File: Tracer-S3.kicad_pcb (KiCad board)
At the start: 2 copper layers, 92.7 x 86.8 mm, 41 parts, among them J1 Conn_01x06_Socket, J2 Conn_02x02_Odd_Even, J3 Conn_02x02_Odd_Even, J4 Conn_02x02_Odd_Even, J5 Conn_02x02_Odd_Even, J6 Conn_02x04_Odd_Even, J7 Conn_01x02_Pin, Q1 BSP89, SW1 SW_Push, SW2 SW_Push, SW3 SW_SPDT, U1 ESP32-S3-WROOM-1, U2 AMS1117-3.3

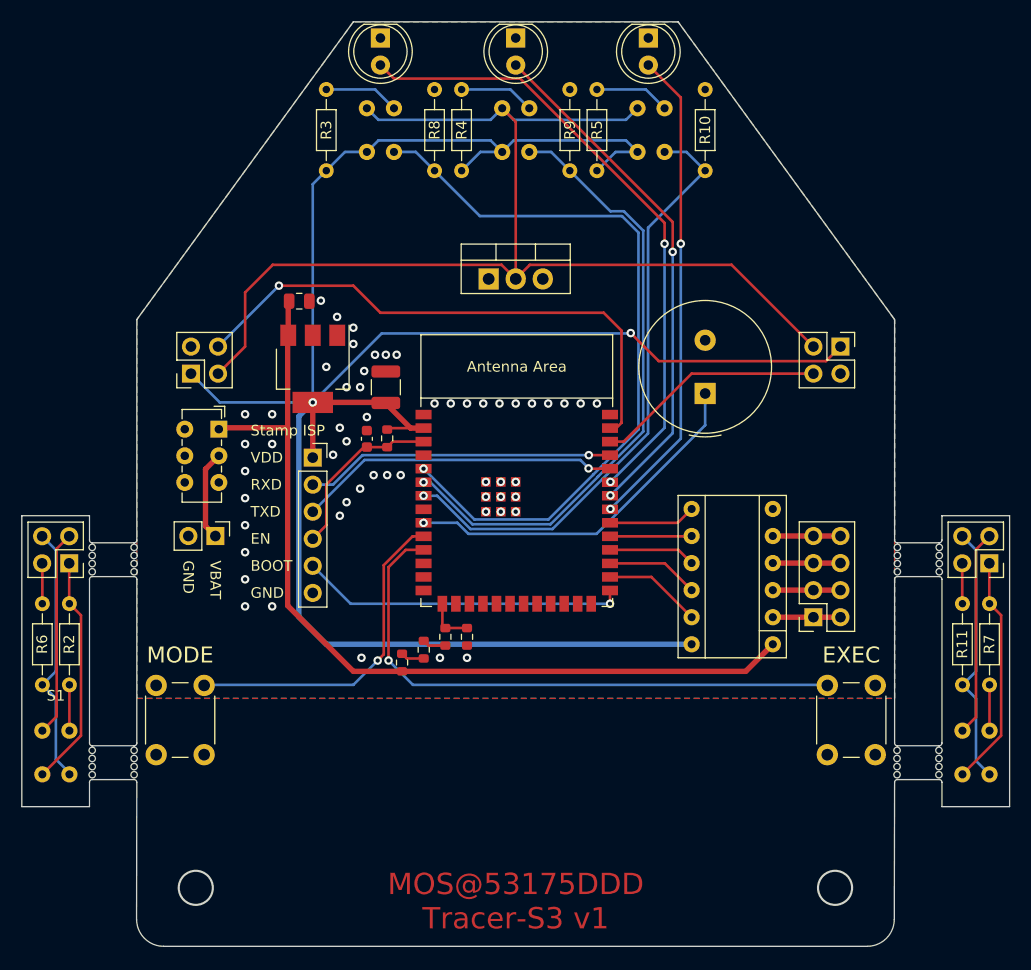
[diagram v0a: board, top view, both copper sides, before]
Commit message: v2
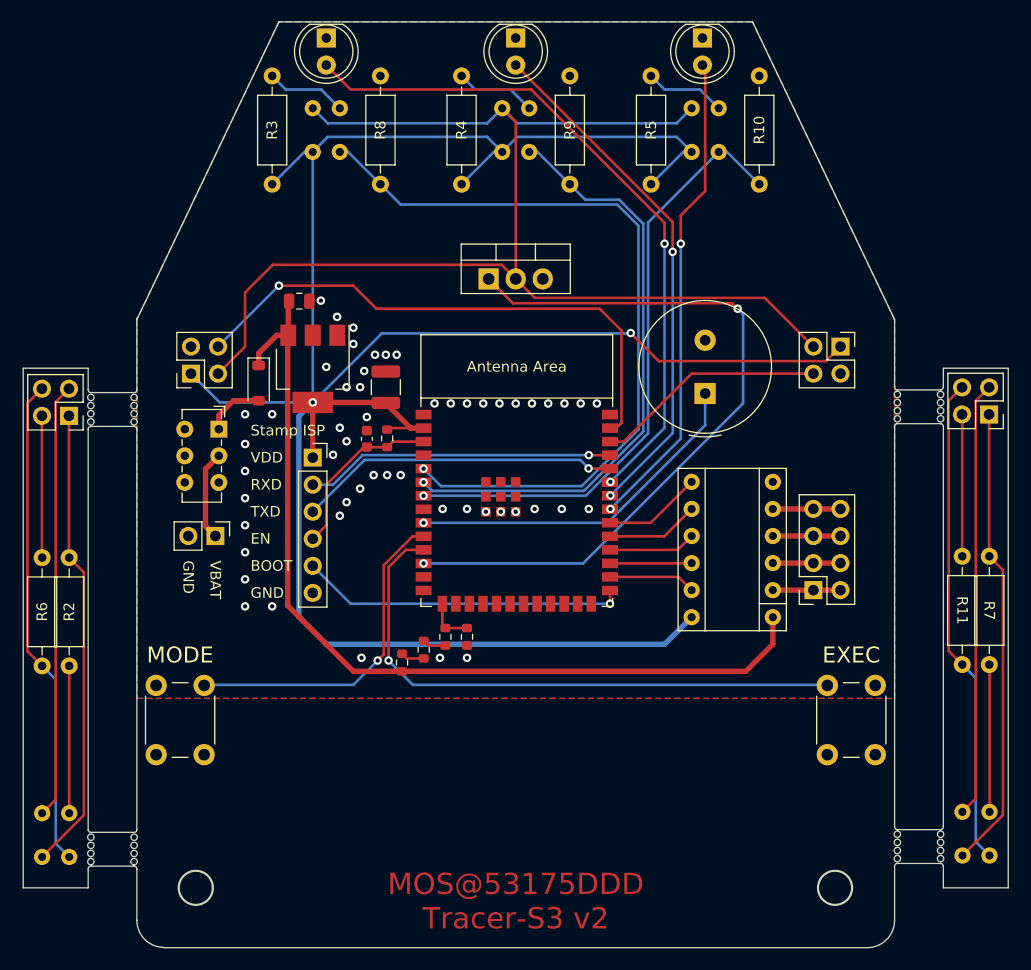
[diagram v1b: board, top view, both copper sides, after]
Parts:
- added D4: D_Schottky, Diode_SMD:D_SOD-123, F.Cu at (128.3, 77.1)
- R10, R11, R2, R3, R4, R5, R6, R7, R8, R9: footprint Resistor_THT:R_Axial_DIN0204_L3.6mm_D1.6mm_P7.62mm_Horizontal -> Resistor_THT:R_Axial_DIN0207_L6.3mm_D2.5mm_P10.16mm_Horizontal
- moved J3 14.0 mm to (196.8, 80.0)
- moved J2 13.8 mm to (110.5, 80.2)
- moved S1 7.75 mm to (109.2, 119.5)
- moved S5 7.62 mm to (195.6, 119.4)
- moved R3 5.24 mm to (129.5, 48.3)
- moved R8 5.24 mm to (139.7, 48.3)
- moved R10 5.24 mm to (175.3, 48.3)
- moved R5 5.24 mm to (165.1, 48.3)
- moved S4 5.08 mm to (170.2, 53.3)
- moved D1 5.08 mm to (134.6, 44.7)
- moved D3 5.08 mm to (169.9, 44.7)
- moved S2 5.08 mm to (134.6, 53.3)
- moved R11 4.45 mm to (194.3, 93.3)
- moved R6 4.32 mm to (108.0, 93.5)
- moved J6 2.54 mm to (180.3, 96.5)
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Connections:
- Q1 pad 1: unconnected-(Q1-G-Pad1) -> /FET_GATE
- SW3 pad 1: +BATT -> Net-(D4-A)
- U1 pad 12: unconnected-(U1-GPIO8/TOUCH8/ADC1_CH7/SUBSPICS1-Pad12) -> /FET_GATE
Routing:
- net /FET_GATE: track 0.00 -> 69.8 mm, vias 0 -> 2
- net +3.3V: track 251.8 -> 309.9 mm
- net /FET_D: track 149.7 -> 202.5 mm
- net /S5: track 46.2 -> 67.8 mm
- net /S1: track 76.4 -> 97.9 mm
- net GND: track 7.60 -> 26.9 mm, vias 55 -> 53
- net Net-(S1-Anode): track 4.30 -> 13.9 mm
- net Net-(S5-Anode): track 4.30 -> 13.8 mm
- net Net-(D4-A): track 0.00 -> 5.61 mm
- net /LED1: track 59.2 -> 64.3 mm
- net /S2: track 70.2 -> 73.1 mm
- net /S3: track 58.5 -> 56.3 mm
- net /MODE: track 9.23 -> 8.17 mm
- net /BIN2: track 8.20 -> 9.25 mm
- net /BIN1: track 7.67 -> 8.72 mm
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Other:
- board size 92.7 x 86.8 mm -> 92.5 x 86.9 mm
- board text added: "MOS@53175DDD Tracer-S3 v2"
- board text removed: "MOS@53175DDD Tracer-S3 v1"
